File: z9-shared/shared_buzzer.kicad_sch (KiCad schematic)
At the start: 6 parts, among them Q701 AO3400A

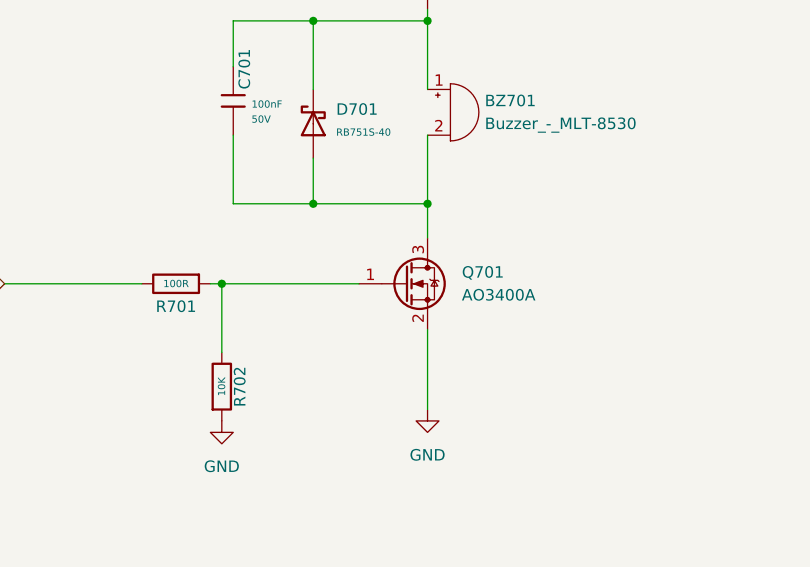
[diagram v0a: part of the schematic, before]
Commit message: more change - generarte jlc
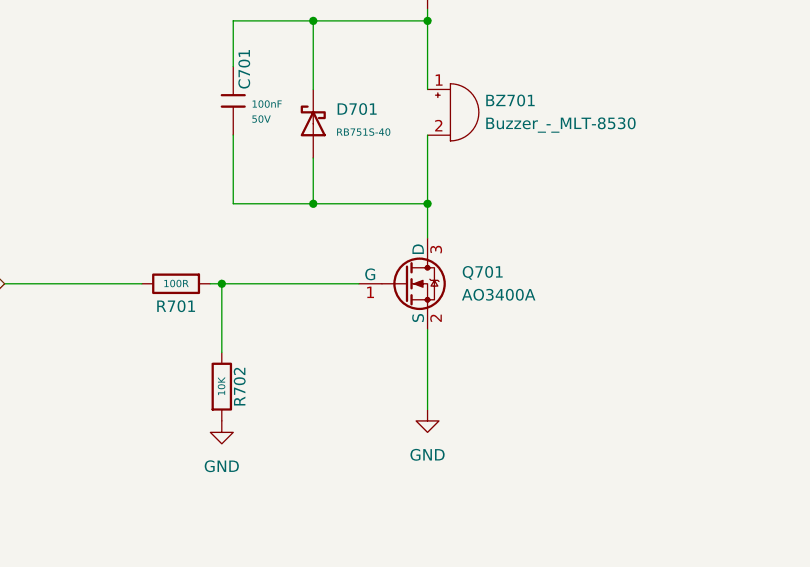
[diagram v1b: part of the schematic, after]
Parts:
- Q701: footprint Package_TO_SOT_SMD:SOT-23 -> PCM_JLCPCB:Q_SOT-23; symbol dnt_global:AO3400A -> PCM_JLCPCB-Transistors:NMOS,AO3400A; Attrition Qty (none) -> 4; Category (none) -> Transistors,MOSFETs; Class (none) -> Basic Component; Continuous Drain Current (Id) (none) -> 5.7A; Drain Source On Resistance (RDS(on)@Vgs,Id) (none) -> 26.5mΩ@10V,5.7A; Drain Source Voltage (Vdss) (none) -> 30V; Gate Threshold Voltage (Vgs(th)@Id) (none) -> 1.5V@250uA; Input Capacitance (Ciss@Vds) (none) -> 630pF@15V; LCSC C2480 -> C20917; Manufacturer (none) -> Alpha & Omega Semicon; Minimum Qty (none) -> 5; Operating Temperature (none) -> -55°C~+150°C@(Tj); Part (none) -> AO3400A; Power Dissipation (Pd) (none) -> 1.4W; Price (none) -> 0.074USD; Process (none) -> SMT; Stock (none) -> 463122; Total Gate Charge (Qg@Vgs) (none) -> 7nC@4.5V; Type (none) -> 1 N-channel
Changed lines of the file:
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@@
 	)
 	(symbol
-		(lib_id "dnt_global:AO3400A")
+		(lib_id "PCM_JLCPCB-Transistors:NMOS,AO3400A")
 		(at 147.32 99.06 0)
 		(unit 1)
@@
 			)
 		)
-		(property "Footprint" "Package_TO_SOT_SMD:SOT-23"
-			(at 152.4 97.155 0)
-			(effects
-				(font
-					(size 1.27 1.27)
-					(italic yes)
-				)
-				(justify left)
-				(hide yes)
-			)
-		)
-		(property "Datasheet" "http://www.aosmd.com/pdfs/datasheet/AO3400A.pdf"
-			(at 152.4 95.25 0)
-			(effects
-				(font
-					(size 1.27 1.27)
-				)
-				(justify left)
-				(hide yes)
-			)
-		)
-		(property "Description" "30V Vds, 5.7A Id, N-Channel MOSFET, SOT-23"
-			(at 147.32 99.06 0)
-			(effects
-				(font
-					(size 1.27 1.27)
-				)
-				(hide yes)
-			)
-		)
-		(property "LCSC" "C2480"
-			(at 147.32 99.06 0)
-			(effects
-				(font
-					(size 1.27 1.27)
-				)
-				(hide yes)
-			)
-		)
-		(property "Order" ""
-			(at 147.32 99.06 0)
-			(effects
-				(font
-					(size 1.27 1.27)
-				)
-				(hide yes)
-			)
-		)
-		(property "PN" ""
-			(at 147.32 99.06 0)
-			(effects
-				(font
-					(size 1.27 1.27)
-				)
-				(hide yes)
-			)
-		)
-		(property "Part Number" ""
-			(at 147.32 99.06 0)
-			(effects
-				(font
-					(size 1.27 1.27)
-				)
-				(hide yes)
-			)
-		)
-		(property "Part#" ""
-			(at 147.32 99.06 0)
-			(effects
-				(font
-					(size 1.27 1.27)
-				)
-				(hide yes)
-			)
-		)
-		(property "Vendor" ""
-			(at 147.32 99.06 0)
-			(effects
-				(font
-					(size 1.27 1.27)
-				)
-				(hide yes)
-			)
-		)
-		(property "Voltage" ""
-			(at 147.32 99.06 0)
-			(effects
+		(property "Footprint" "PCM_JLCPCB:Q_SOT-23"
+			(at 145.542 99.06 90)
+			(effects
+				(font
+					(size 1.27 1.27)
+				)
+				(hide yes)
+			)
+		)
+		(property "Datasheet" "https://www.lcsc.com/datasheet/lcsc_datasheet_1811081213_Alpha---Omega-Semicon-AO3400A_C20917.pdf"
+			(at 147.32 99.06 0)
+			(effects
+				(font
+					(size 1.27 1.27)
+				)
+				(hide yes)
+			)
+		)
+		(property "Description" "30V 5.7A 26.5mΩ@10V,5.7A 1.4W 1.5V@250uA 1 N-Channel SOT-23-3L MOSFETs ROHS"
+			(at 147.32 99.06 0)
+			(effects
+				(font
+					(size 1.27 1.27)
+				)
+				(hide yes)
+			)
+		)
+		(property "LCSC" "C20917"
+			(at 147.32 99.06 0)
+			(effects
+				(font
+					(size 1.27 1.27)
+				)
+				(hide yes)
+			)
+		)
+		(property "Stock" "463122"
+			(at 147.32 99.06 0)
+			(effects
+				(font
+					(size 1.27 1.27)
+				)
+				(hide yes)
+			)
+		)
+		(property "Price" "0.074USD"
+			(at 147.32 99.06 0)
+			(effects
+				(font
+					(size 1.27 1.27)
+				)
+				(hide yes)
+			)
+		)
+		(property "Process" "SMT"
+			(at 147.32 99.06 0)
+			(effects
+				(font
+					(size 1.27 1.27)
+				)
+				(hide yes)
+			)
+		)
+		(property "Minimum Qty" "5"
+			(at 147.32 99.06 0)
+			(effects
+				(font
+					(size 1.27 1.27)
+				)
+				(hide yes)
+			)
+		)
+		(property "Attrition Qty" "4"
+			(at 147.32 99.06 0)
+			(effects
+				(font
+					(size 1.27 1.27)
+				)
+				(hide yes)
+			)
+		)
+		(property "Class" "Basic Component"
+			(at 147.32 99.06 0)
+			(effects
+				(font
+					(size 1.27 1.27)
+				)
+				(hide yes)
+			)
+		)
+		(property "Category" "Transistors,MOSFETs"
+			(at 147.32 99.06 0)
+			(effects
+				(font
+					(size 1.27 1.27)
+				)
+				(hide yes)
+			)
+		)
+		(property "Manufacturer" "Alpha & Omega Semicon"
+			(at 147.32 99.06 0)
+			(effects
+				(font
+					(size 1.27 1.27)
+				)
+				(hide yes)
+			)
+		)
+		(property "Part" "AO3400A"
+			(at 147.32 99.06 0)
+			(effects
+				(font
+					(size 1.27 1.27)
+				)
+				(hide yes)
+			)
+		)
+		(property "Continuous Drain Current (Id)" "5.7A"
+			(at 147.32 99.06 0)
+			(effects
+				(font
+					(size 1.27 1.27)
+				)
+				(hide yes)
+			)
+		)
+		(property "Input Capacitance (Ciss@Vds)" "630pF@15V"
+			(at 147.32 99.06 0)
+			(effects
+				(font
+					(size 1.27 1.27)
+				)
+				(hide yes)
+			)
+		)
+		(property "Operating Temperature" "-55°C~+150°C@(Tj)"
+			(at 147.32 99.06 0)
+			(effects
+				(font
+					(size 1.27 1.27)
+				)
+				(hide yes)
+			)
+		)
+		(property "Type" "1 N-channel"
+			(at 147.32 99.06 0)
+			(effects
+				(font
+					(size 1.27 1.27)
+				)
+				(hide yes)
+			)
+		)
+		(property "Drain Source Voltage (Vdss)" "30V"
+			(at 147.32 99.06 0)
+			(effects
+				(font
+					(size 1.27 1.27)
+				)
+				(hide yes)
+			)
+		)
+		(property "Power Dissipation (Pd)" "1.4W"
+			(at 147.32 99.06 0)
+			(effects
+				(font
+					(size 1.27 1.27)
+				)
+				(hide yes)
+			)
+		)
+		(property "Gate Threshold Voltage (Vgs(th)@Id)" "1.5V@250uA"
+			(at 147.32 99.06 0)
+			(effects
+				(font
+					(size 1.27 1.27)
+				)
+				(hide yes)
+			)
+		)
+		(property "Drain Source On Resistance (RDS(on)@Vgs,Id)" "26.5mΩ@10V,5.7A"
+			(at 147.32 99.06 0)
+			(effects
+				(font
+					(size 1.27 1.27)
+				)
+				(hide yes)
+			)
+		)
+		(property "Total Gate Charge (Qg@Vgs)" "7nC@4.5V"
+			(at 147.32 99.06 0)
+			(effects

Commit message: more moving offset to library - tedious
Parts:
- BZ701: FT Rotation Offset (none) -> -90
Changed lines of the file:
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@@
 			)
 		)
-		(property "Order" ""
+		(property "FT Rotation Offset" "-90"
 			(at 152.4 80.01 0)
 			(effects
-				(font
-					(size 1.27 1.27)
-				)
-				(hide yes)
-			)
-		)
-		(property "PN" ""
-			(at 152.4 80.01 0)
-			(effects
-				(font
-					(size 1.27 1.27)
-				)
-				(hide yes)
-			)
-		)
-		(property "Part Number" ""
-			(at 152.4 80.01 0)
-			(effects
-				(font
-					(size 1.27 1.27)
-				)
-				(hide yes)
-			)
-		)
-		(property "Part#" ""
-			(at 152.4 80.01 0)
-			(effects
-				(font
-					(size 1.27 1.27)
-				)
-				(hide yes)
-			)
-		)
-		(property "Vendor" ""
-			(at 152.4 80.01 0)
-			(effects
-				(font
-					(size 1.27 1.27)
-				)
-				(hide yes)
-			)
-		)
-		(property "Voltage" ""
-			(at 152.4 80.01 0)
-			(effects

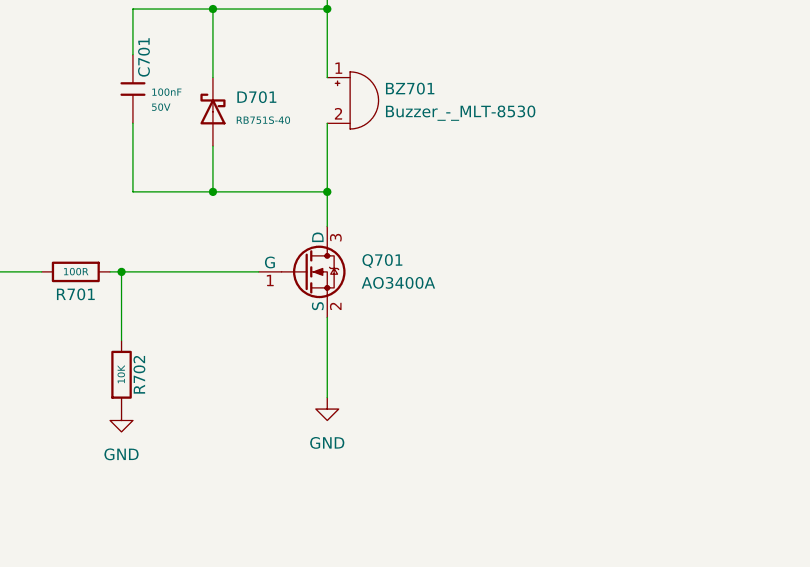
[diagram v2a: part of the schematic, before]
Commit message: ism issues
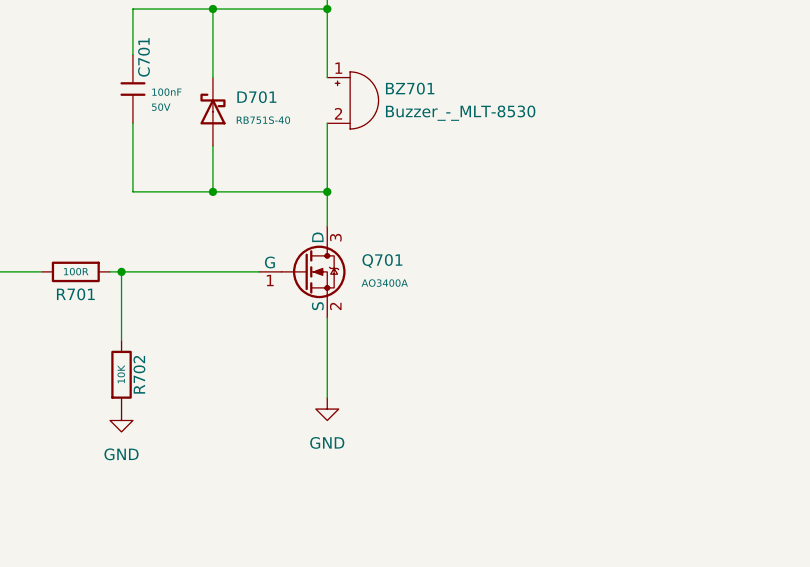
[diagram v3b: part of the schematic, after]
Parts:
- Q701: symbol PCM_JLCPCB-Transistors:NMOS,AO3400A -> dnt_global:NMOS,AO3400A; FT Rotation Offset (none) -> 180
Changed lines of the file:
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@@
 	)
 	(symbol
-		(lib_id "PCM_JLCPCB-Transistors:NMOS,AO3400A")
+		(lib_id "dnt_global:NMOS,AO3400A")
 		(at 147.32 99.06 0)
 		(unit 1)
@@
 		)
 		(property "Value" "AO3400A"
-			(at 153.67 100.3299 0)
-			(effects
-				(font
-					(size 1.27 1.27)
+			(at 153.67 100.33 0)
+			(effects
+				(font
+					(size 0.8 0.8)
 				)
 				(justify left)
@@
 			(at 147.32 99.06 0)
 			(effects
+				(font
+					(size 1.27 1.27)
+				)
+				(hide yes)
+			)
+		)
+		(property "FT Rotation Offset" "180"
+			(at 147.32 99.06 0)
+			(effects
